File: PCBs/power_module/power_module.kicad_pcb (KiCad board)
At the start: 2 copper layers, 38.8 x 38.8 mm, 34 parts, among them J1 Conn_02x07_Odd_Even, J2 Conn_02x08_Odd_Even, J3 Conn_02x08_Odd_Even, J4 SM07B-GHS-TB, J5 SM03B-GHS-TB, J6 SM02B-GHS-TB, J7 SM08B-GHS-TB, U1 SN74LVC1T45DBV

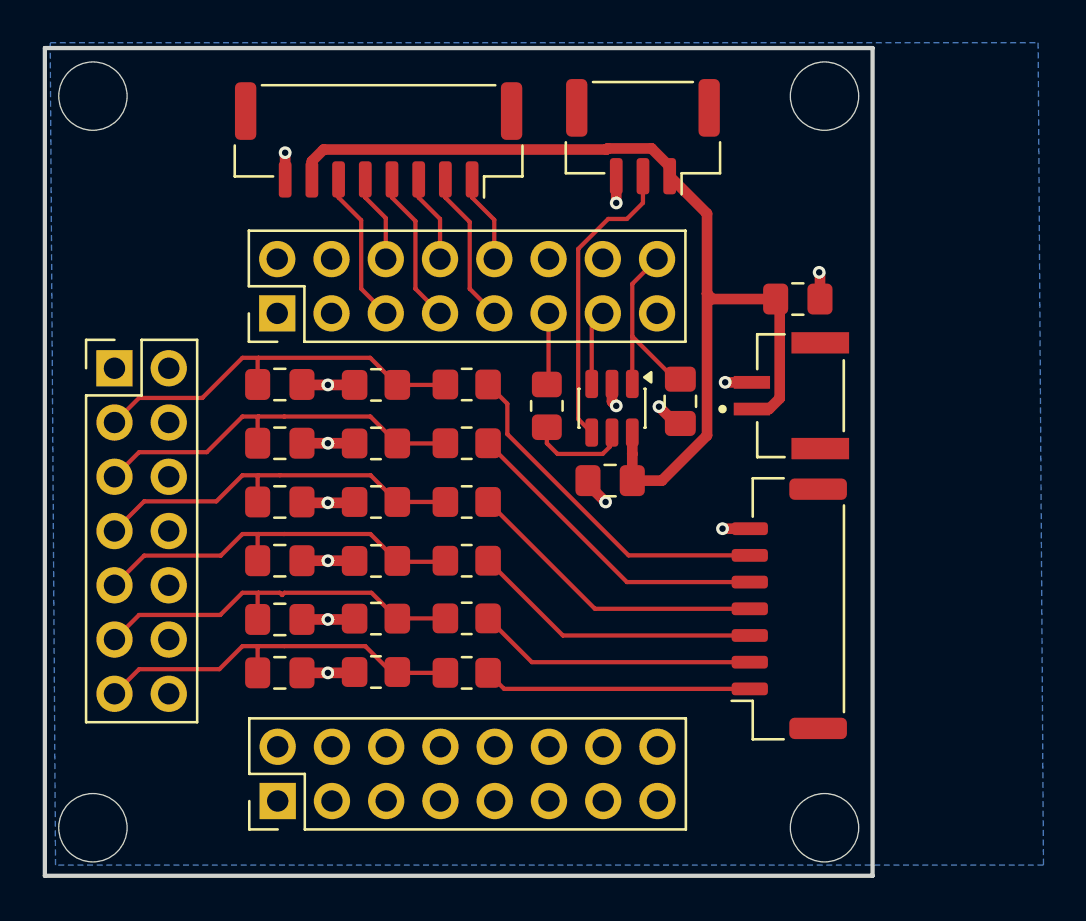
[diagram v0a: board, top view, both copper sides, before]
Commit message: cleaned up folders
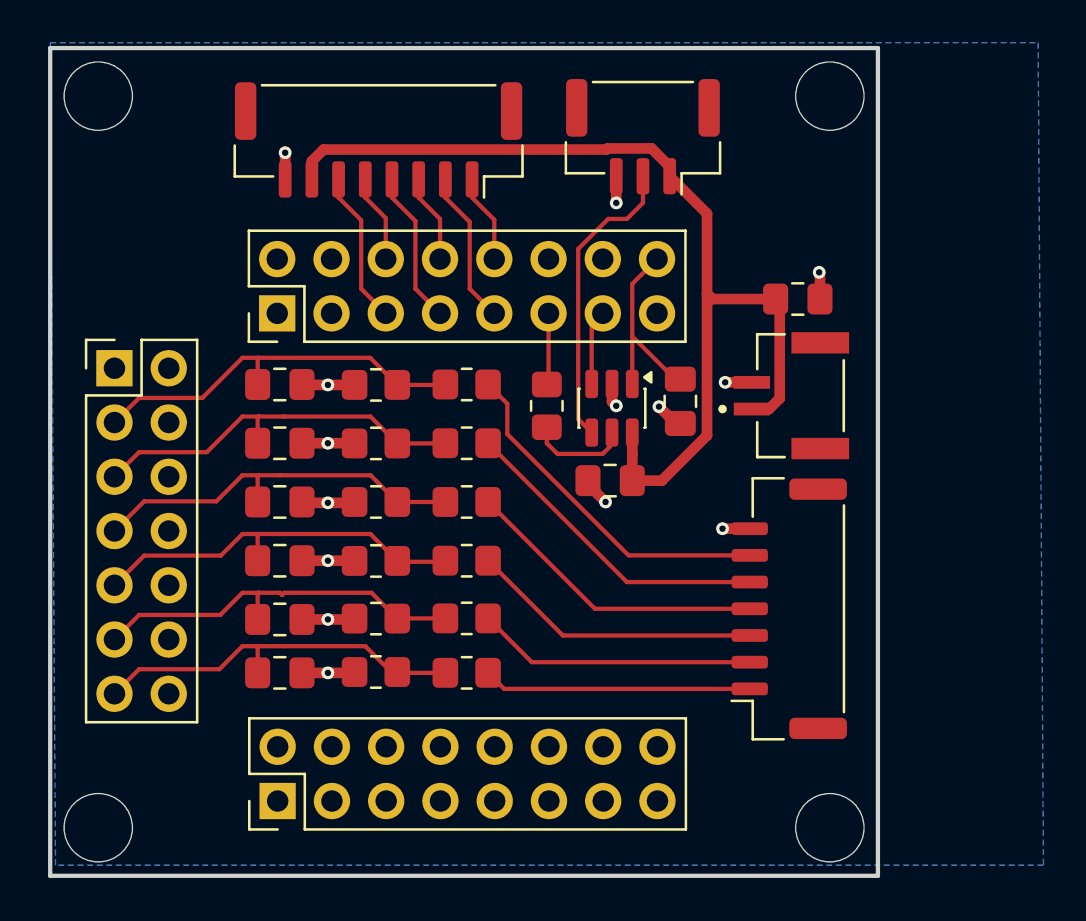
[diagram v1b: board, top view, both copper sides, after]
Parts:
- moved H1 0.25 mm to (125.5, 46.5)
- moved H2 0.25 mm to (125.5, 80.8)
- moved H3 0.25 mm to (159.8, 46.5)
- moved H4 0.25 mm to (159.8, 80.8)
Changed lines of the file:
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@@
 		)
 		(embedded_fonts no)
-		(model "${KIPRJMOD}/SM02B_GHS_TB/SM02B-GHS-TB.step"
+		(model "${KIPRJMOD}/imported_connector_files/SM02B_GHS_TB/SM02B-GHS-TB.step"
 			(offset
 				(xyz 0 -0.3 0)
@@
 	(footprint "MountingHole:MountingHole_3.2mm_M3"
 		(layer "F.Cu")
-		(at 159.5 46.5)
+		(at 159.75 46.5)
 		(descr "Mounting Hole 3.2mm, M3, no annular, generated by kicad-footprint-generator mountinghole.py")
 		(tags "mountinghole M3")
@@
 	(footprint "MountingHole:MountingHole_3.2mm_M3"
 		(layer "F.Cu")
-		(at 125.25 46.5)
+		(at 125.5 46.5)
 		(descr "Mounting Hole 3.2mm, M3, no annular, generated by kicad-footprint-generator mountinghole.py")
 		(tags "mountinghole M3")
@@
 	(footprint "MountingHole:MountingHole_3.2mm_M3"
 		(layer "F.Cu")
-		(at 125.25 80.75)
+		(at 125.5 80.75)
 		(descr "Mounting Hole 3.2mm, M3, no annular, generated by kicad-footprint-generator mountinghole.py")
 		(tags "mountinghole M3")
@@
 	(footprint "MountingHole:MountingHole_3.2mm_M3"
 		(layer "F.Cu")
-		(at 159.5 80.75)
+		(at 159.75 80.75)
 		(descr "Mounting Hole 3.2mm, M3, no annular, generated by kicad-footprint-generator mountinghole.py")
 		(tags "mountinghole M3")
@@
 	)
 	(gr_rect
-		(start 123 44.25)
-		(end 161.75 83)
+		(start 123.25 44.25)
+		(end 162 83)
 		(stroke
 			(width 0.2)
@@
 	)
 	(gr_text "5V In"
-		(at 163.5 66.75 90)
+		(at 163.75 62.25 90)
 		(layer "Cmts.User")
 		(effects
@@
 	)
 	(gr_text "Battery In\n"
-		(at 163.25 78.5 90)
+		(at 163.75 74 90)
 		(layer "Cmts.User")
 		(effects
@@
 	)
 	(gr_text "Relays Out"
-		(at 134.75 43.75 0)
+		(at 134.25 43.75 0)
 		(layer "Cmts.User")
 		(effects
@@
 	)
 	(gr_text "Level Shifter Out"
-		(at 145 43.75 0)
+		(at 144.5 43.75 0)
 		(layer "Cmts.User")
 		(effects
@@
 		(layer "Dwgs.User")
 		(pts
-			(xy 123 44.25) (xy 123 83)
+			(xy 123.25 44.25) (xy 123.25 83)
 		)
 		(height -4.5)
@@
 		)
 		(gr_text "38.7500 mm"
-			(at 117.35 63.625 90)
+			(at 117.6 63.625 90)
 			(layer "Dwgs.User")
 			(effects
@@
 		(layer "Dwgs.User")
 		(pts
-			(xy 123 83) (xy 161.75 83)
+			(xy 123.25 83) (xy 162 83)
 		)
 		(height 6.75)
@@
 		)
 		(gr_text "38.7500 mm"
-			(at 142.375 88.6 0)
+			(at 142.625 88.6 0)
 			(layer "Dwgs.User")
 			(effects
